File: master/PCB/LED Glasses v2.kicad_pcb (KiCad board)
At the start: 2 copper layers, 152.9 x 54.6 mm, 85 parts, among them J1 Conn_01x01_Male, J2 Conn_01x01_Male, J3 Conn_01x01_Male, J4 Conn_01x01_Male, J5 Conn_01x01_Male

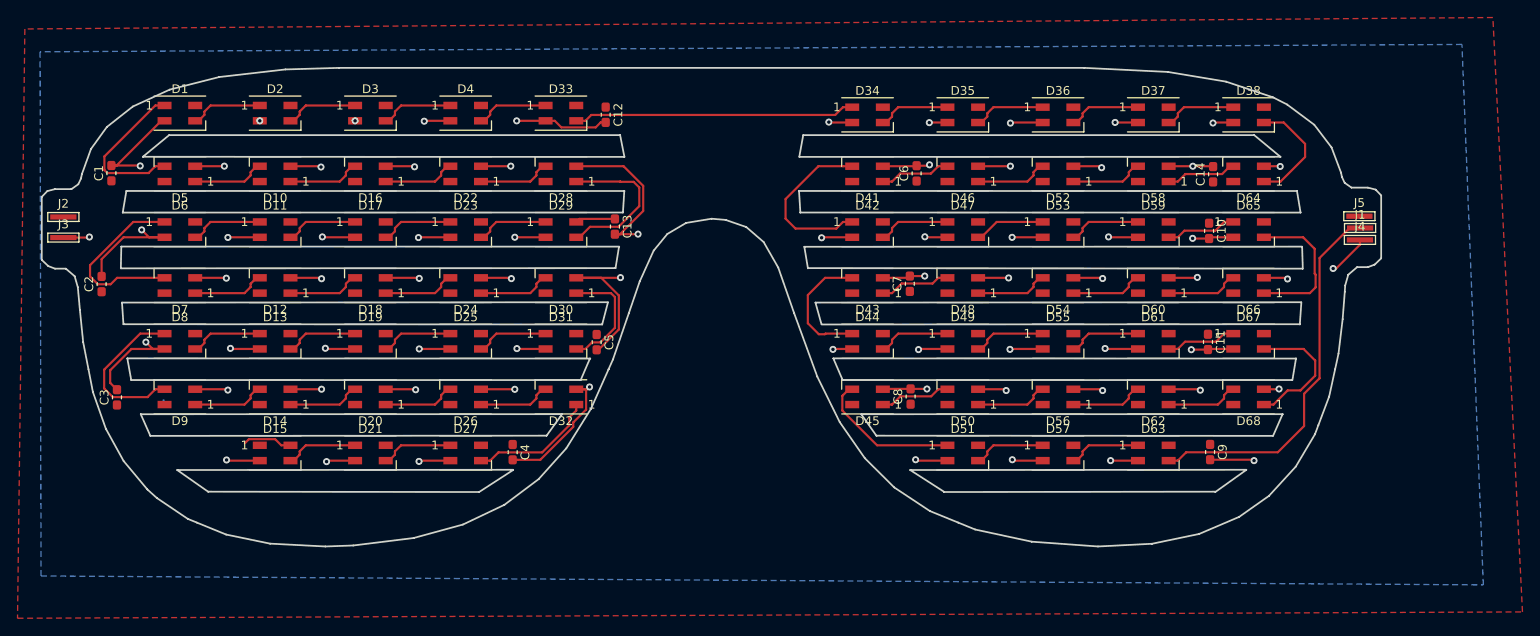
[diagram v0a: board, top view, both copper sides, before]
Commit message: gerber zip
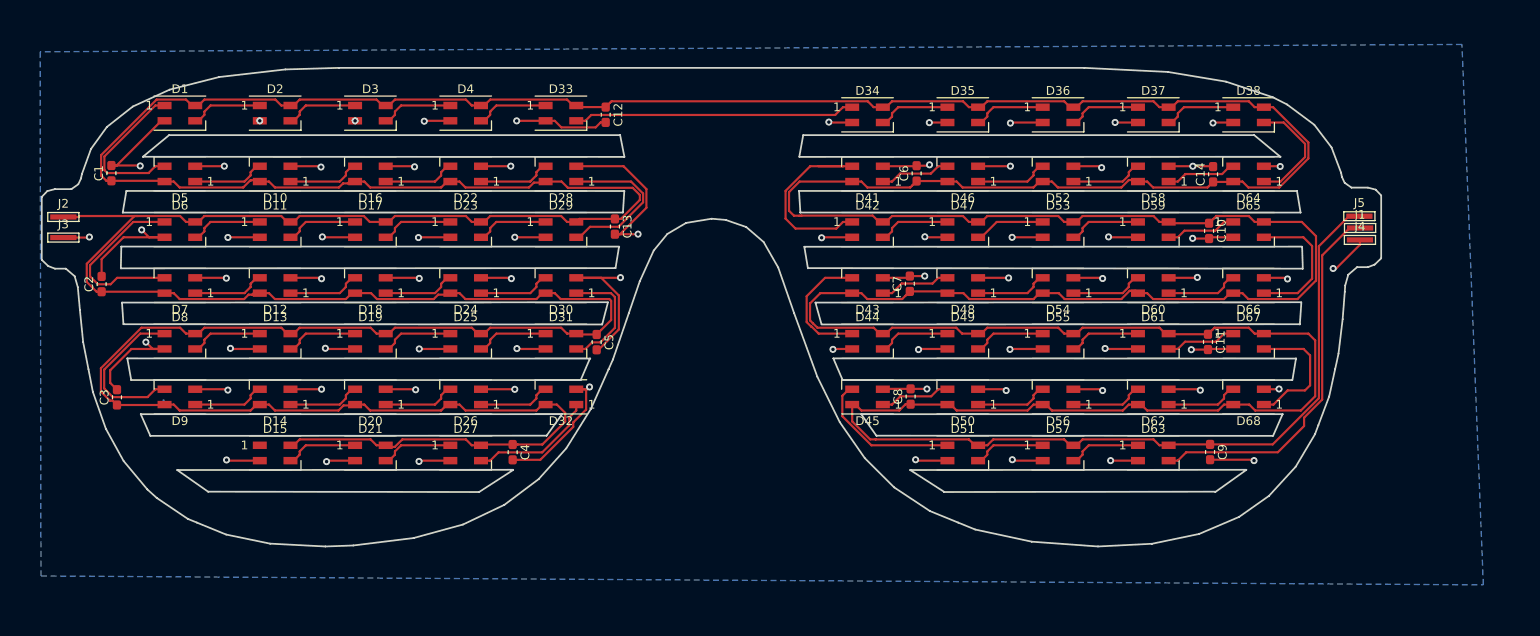
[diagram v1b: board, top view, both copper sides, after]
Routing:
- net Net-(C1-Pad1): track 10.3 -> 924.1 mm
- net Net-(D41-Pad3): track 19.8 -> 23.1 mm
- net Net-(D65-Pad3): track 17.0 -> 15.8 mm
- removed copper zone on F.Cu, net Net-(C1-Pad1)
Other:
- net class Default: clearance 0.2 -> 0.125
- rule trace_clearance: 0.2 -> 0.125
